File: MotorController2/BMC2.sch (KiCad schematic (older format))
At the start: 27 parts, among them P1 Sensor, P10 GND, P11 I2C, P12 CAN, P2 CAN, P3 DATA, P4 USB_OTG, P5 PhaseA, P6 PhaseB, P7 PhaseC, P9 VSUPPLY, U1 TJA1042T/3

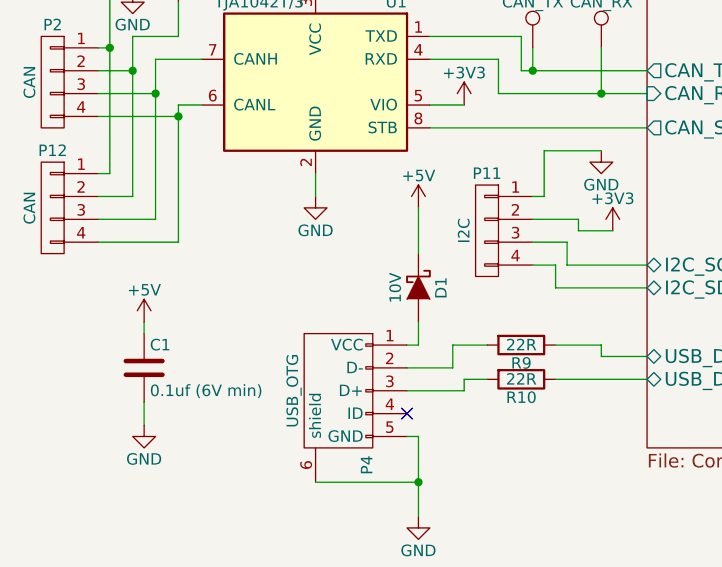
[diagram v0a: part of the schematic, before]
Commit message: Layout nearly complete.
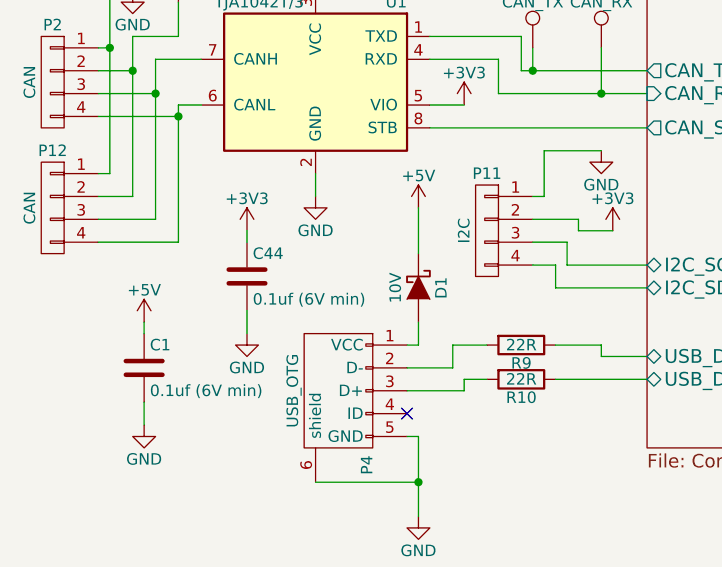
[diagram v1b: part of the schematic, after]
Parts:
- added C44: 0.1uf (6V min), Capacitors_SMD:C_0805_HandSoldering, symbol C
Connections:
- net +3V3: now also C44.1
- net GND: now also C44.2
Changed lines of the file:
@@
 LIBS:IFX91041EJV33
 LIBS:BMC2-cache
-EELAYER 26 0
+EELAYER 25 0
 EELAYER END
 $Descr A4 11693 8268
@@
 Wire Wire Line
 	2800 2950 3350 2950
+$Comp
+L +3V3 #PWR020
+U 1 1 587B9A34
+P 1600 4650
+F 0 "#PWR020" H 1600 4500 50  0001 C CNN
+F 1 "+3V3" H 1600 4790 50  0000 C CNN
+F 2 "" H 1600 4650 50  0000 C CNN
+F 3 "" H 1600 4650 50  0000 C CNN
+	1    1600 4650
+	1    0    0    -1
+$EndComp
+$Comp
+L C C44
+U 1 1 587B9C10
+P 1600 4850
+F 0 "C44" H 1625 4950 50  0000 L CNN
+F 1 "0.1uf (6V min)" H 1625 4750 50  0000 L CNN
+F 2 "Capacitors_SMD:C_0805_HandSoldering" H 1638 4700 50  0001 C CNN
+F 3 "" H 1600 4850 50  0000 C CNN
+	1    1600 4850
+	1    0    0    -1
+$EndComp
+$Comp
+L GND #PWR021
+U 1 1 587B9DFF
+P 1600 5100
+F 0 "#PWR021" H 1600 4850 50  0001 C CNN
+F 1 "GND" H 1600 4950 50  0000 C CNN
+F 2 "" H 1600 5100 50  0000 C CNN
+F 3 "" H 1600 5100 50  0000 C CNN
+	1    1600 5100
+	1    0    0    -1
+$EndComp
+Wire Wire Line
+	1600 5100 1600 5000
+Wire Wire Line
+	1600 4700 1600 4650
 $EndSCHEMATC
